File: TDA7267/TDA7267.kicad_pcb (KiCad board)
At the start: 2 copper layers, 43 x 39 mm, 18 parts, among them U1 TDA7267

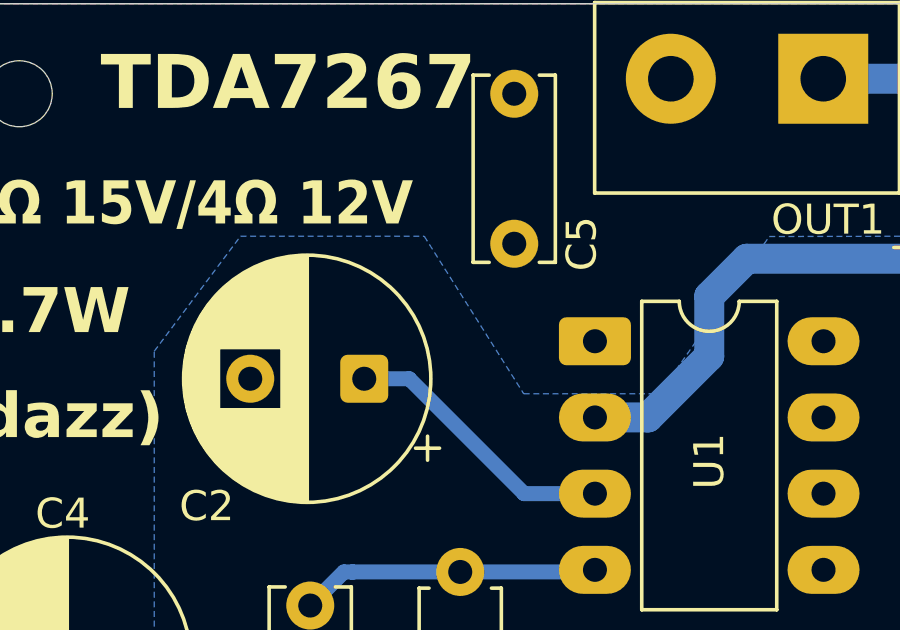
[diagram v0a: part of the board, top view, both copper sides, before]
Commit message: Tweaks
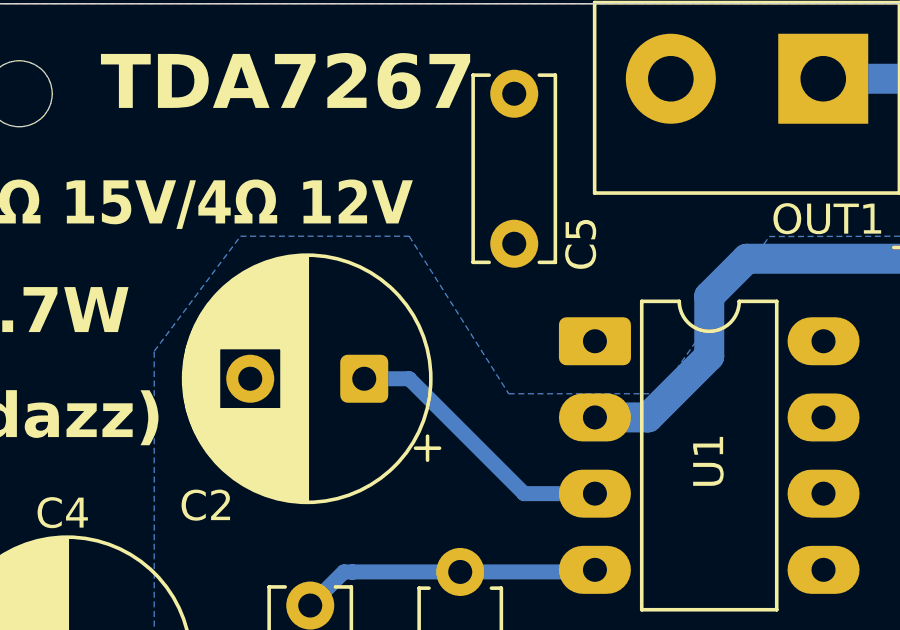
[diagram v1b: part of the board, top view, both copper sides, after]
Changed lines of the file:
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@@
 		(hatch edge 0.5)
 		(connect_pads yes
-			(clearance 0.25)
+			(clearance 0.3)
 		)
 		(min_thickness 0.25)
@@
 		(priority 1)
 		(connect_pads yes
-			(clearance 0.5)
+			(clearance 0.3)
 		)
 		(min_thickness 0.25)
@@
 		(polygon
 			(pts
-				(xy 136.5 117.5) (xy 136.5 90.083326) (xy 139.374995 86.25) (xy 145.5 86.25) (xy 148.81579 91.5)
-				(xy 153.342105 91.5) (xy 157 86.259441) (xy 161.7 86.25) (xy 163 90.607672) (xy 168.293873 94.273373)
-				(xy 168.308026 99.362426) (xy 174 99.344523) (xy 174 117.5)
+				(xy 136.5 117.5) (xy 136.5 90.083326) (xy 139.374995 86.25) (xy 145 86.25) (xy 148.31579 91.5) (xy 153.342105 91.5)
+				(xy 157 86.259441) (xy 161.7 86.25) (xy 163 90.607672) (xy 168.293873 94.273373) (xy 168.308026 99.362426)
+				(xy 174 99.344523) (xy 174 117.5)
 			)
 		)
@@
 		(hatch edge 0.5)
 		(connect_pads yes
-			(clearance 0.5)
+			(clearance 0.3)
 		)
 		(min_thickness 0.25)
